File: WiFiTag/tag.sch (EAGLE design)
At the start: 65 parts, among them IC2 MCP73831/OT, U2 CP2104-F03-GM

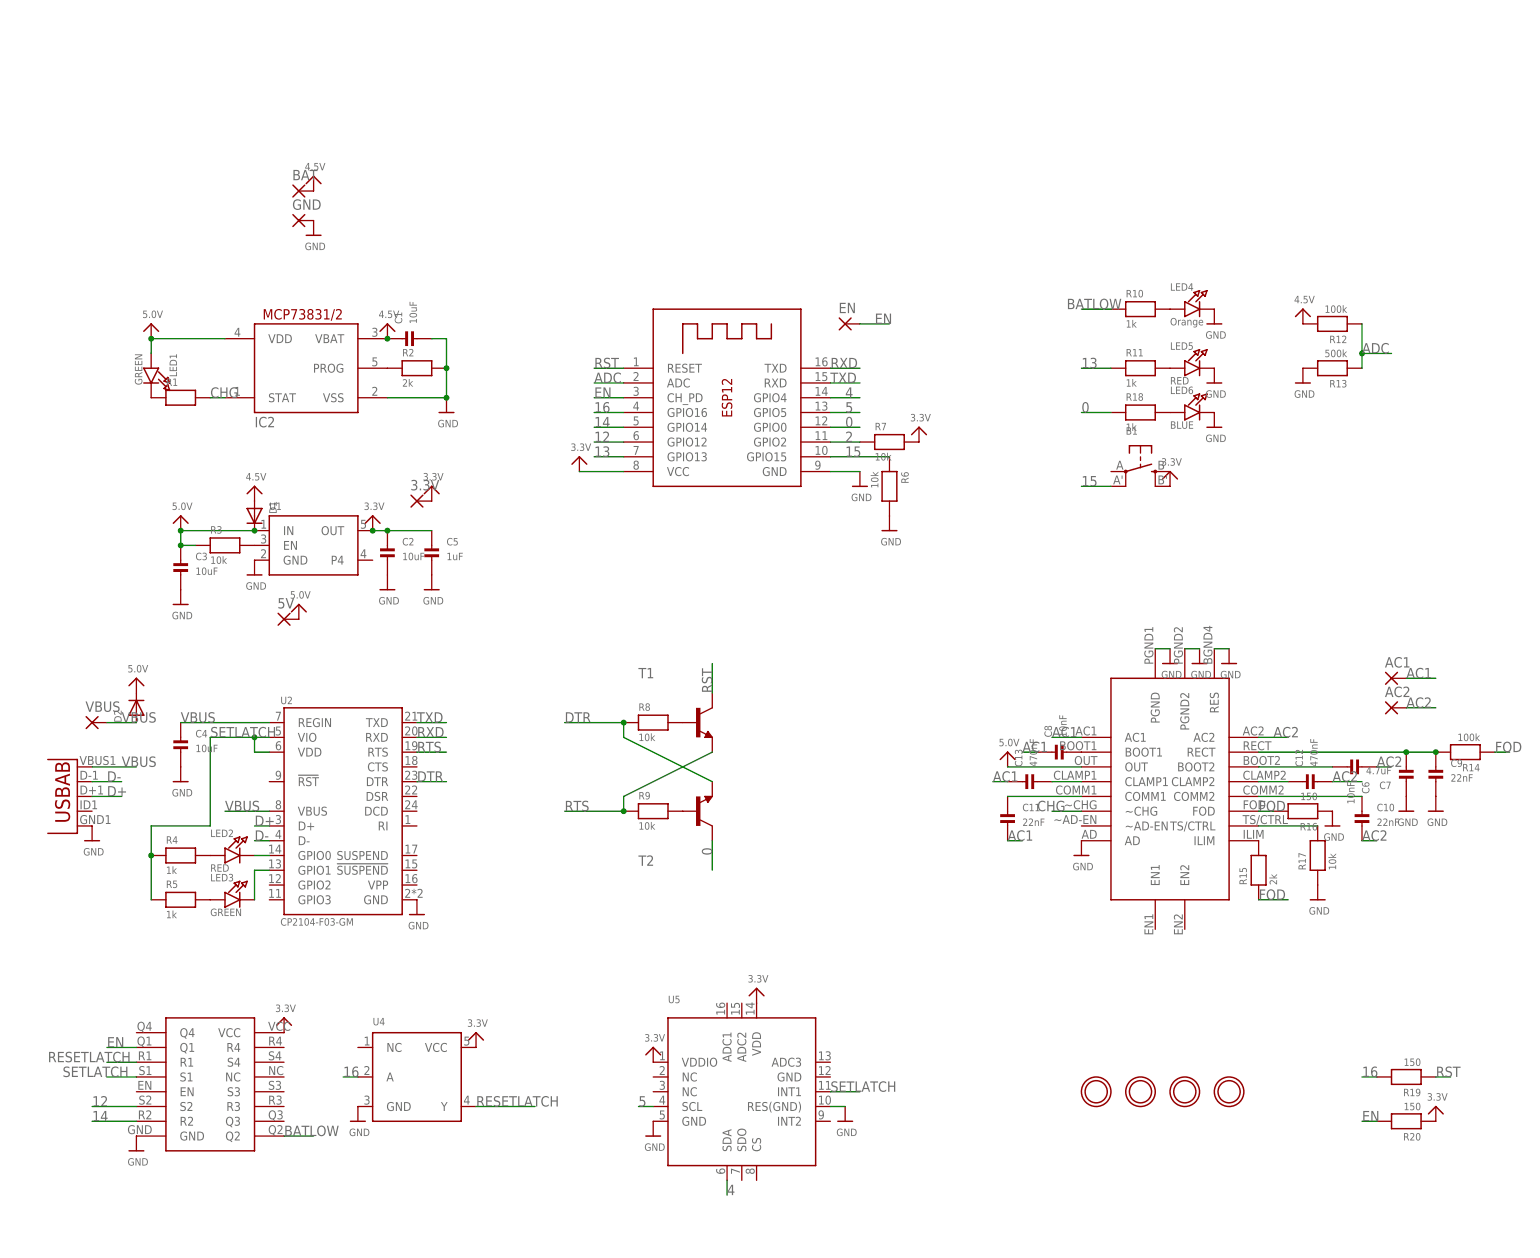
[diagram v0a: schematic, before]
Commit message: WifiTagV0.4
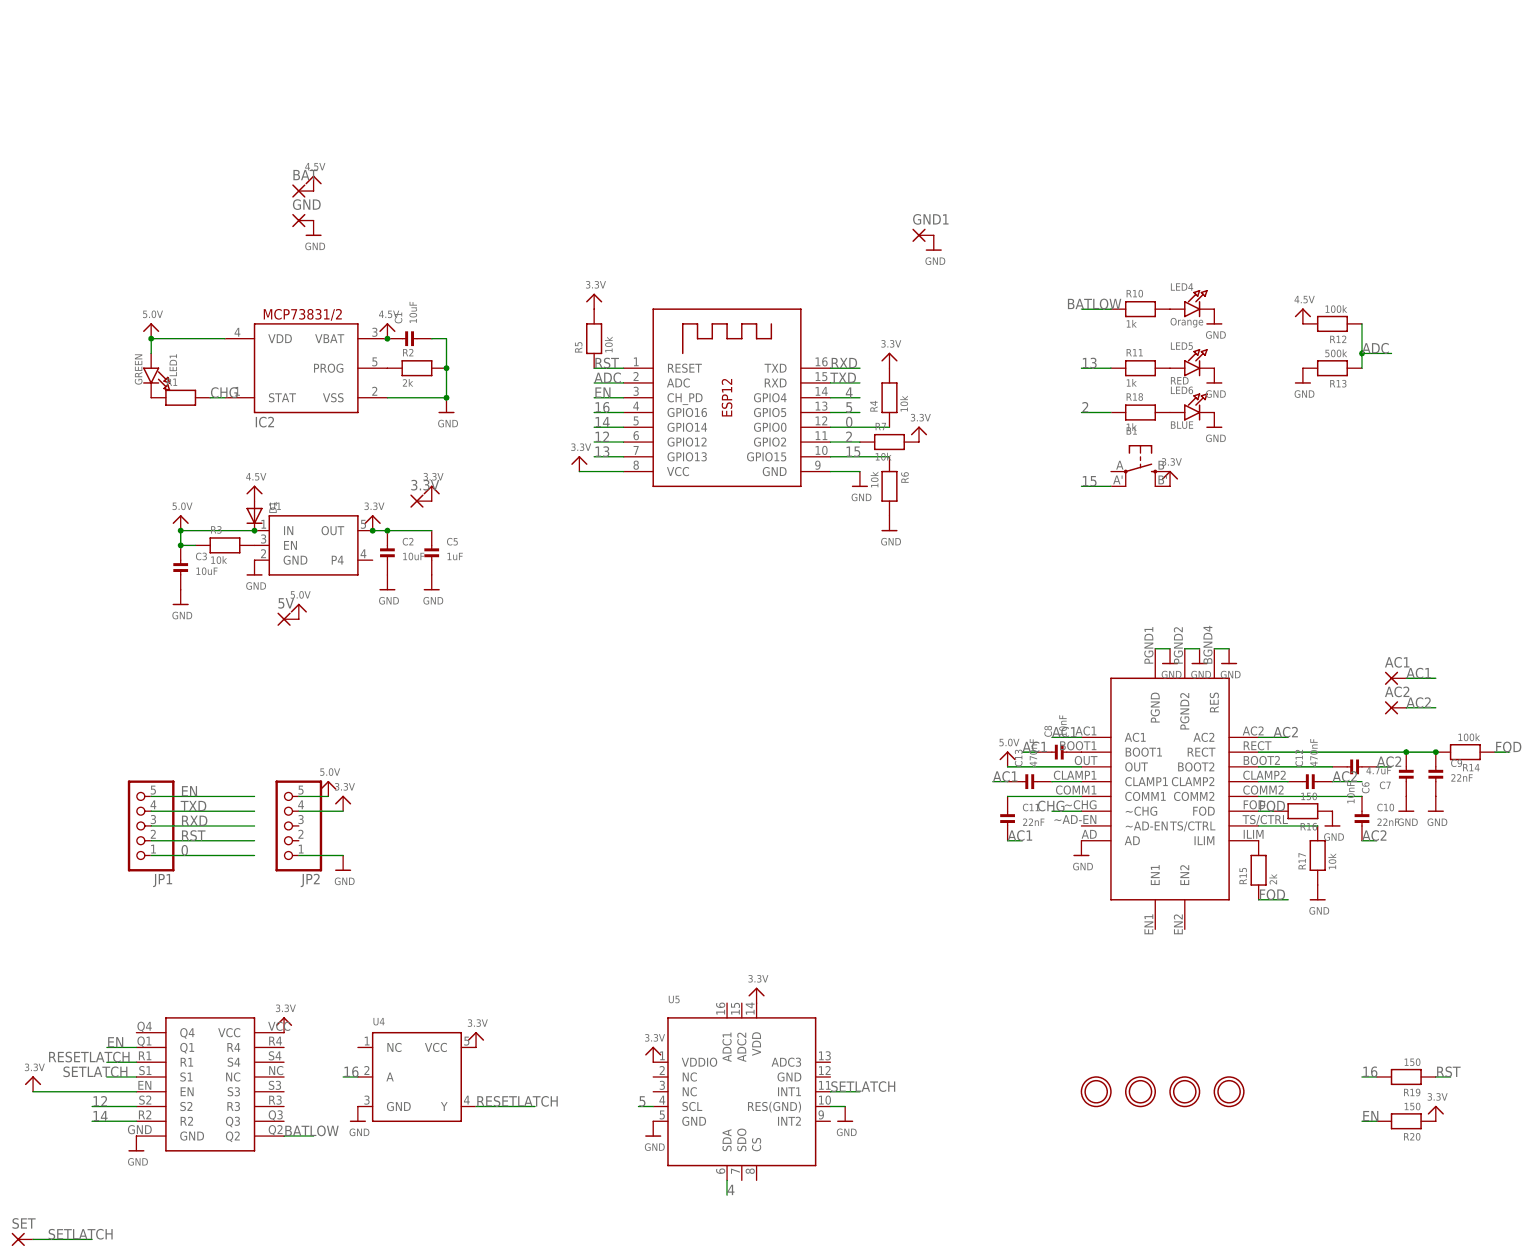
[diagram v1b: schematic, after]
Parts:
- removed C4: 10uF, microbuilder:CAP_CERAMIC0603
- removed D2: (no value), adafruit:DIODESOD-123
- removed EN, VBUS: (no value), wirepad:SMD2
- removed LED2: RED, microbuilder:LED0603
- removed LED3: GREEN, microbuilder:LED0603
- removed R8, R9: 10k, microbuilder:RESISTOR0402
- removed T1, T2: (no value), transistor:MMBT2222ALT1-NPN-SOT23-BEC
- removed U2: CP2104-F03-GM, Silicon Labs:CP2104-F03-GM
- removed U3: (no value), MicroUSB:USB""
- added GND1, SET: (no value), wirepad:SMD2
- added JP1, JP2: (no value), pinhead:PINHD-1X55X2MM
- R4, R5: value 1k -> 10k
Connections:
- removed net D+: U2.D+, U3.D+
- removed net D-: U2.D-, U3.D-
- removed net DTR: R8.1, T2.E, U2.DTR
- removed net N$10: R8.2, T1.B
- removed net N$11: R9.2, T2.B
- removed net N$6: LED2.A, R4.2
- removed net N$7: LED3.A, R5.2
- removed net N$8: LED2.C, U2.GPIO0
- removed net N$9: LED3.C, U2.GPIO1
- removed net RTS: R9.1, T1.E, U2.RTS
- removed net VBUS: C4.P$1, D2.A, U2.REGIN, U2.VBUS, U3.VBUS, VBUS.P
- net 0: now also JP1.1, R4.1; no longer R18.1, T2.C
- net 2: now also R18.1
- net 3.3V: now also JP2.4, R4.2, R5.2, U$24.EN
- net 5.0V: now also JP2.5; no longer D2.C
- net EN: now also JP1.5; no longer EN.P
- net GND: now also GND1.P, JP2.1; no longer C4.P$2, U2.GND, U3.GND
- net RST: now also JP1.2, R5.1; no longer T1.C
- net RXD: now also JP1.3; no longer U2.RXD
- net SETLATCH: now also SET.P; no longer R4.1, R5.1, U2.VDD, U2.VIO
- net TXD: now also JP1.4; no longer U2.TXD
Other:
- moved on the sheet: R4, R5

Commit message: new tag version 0.5
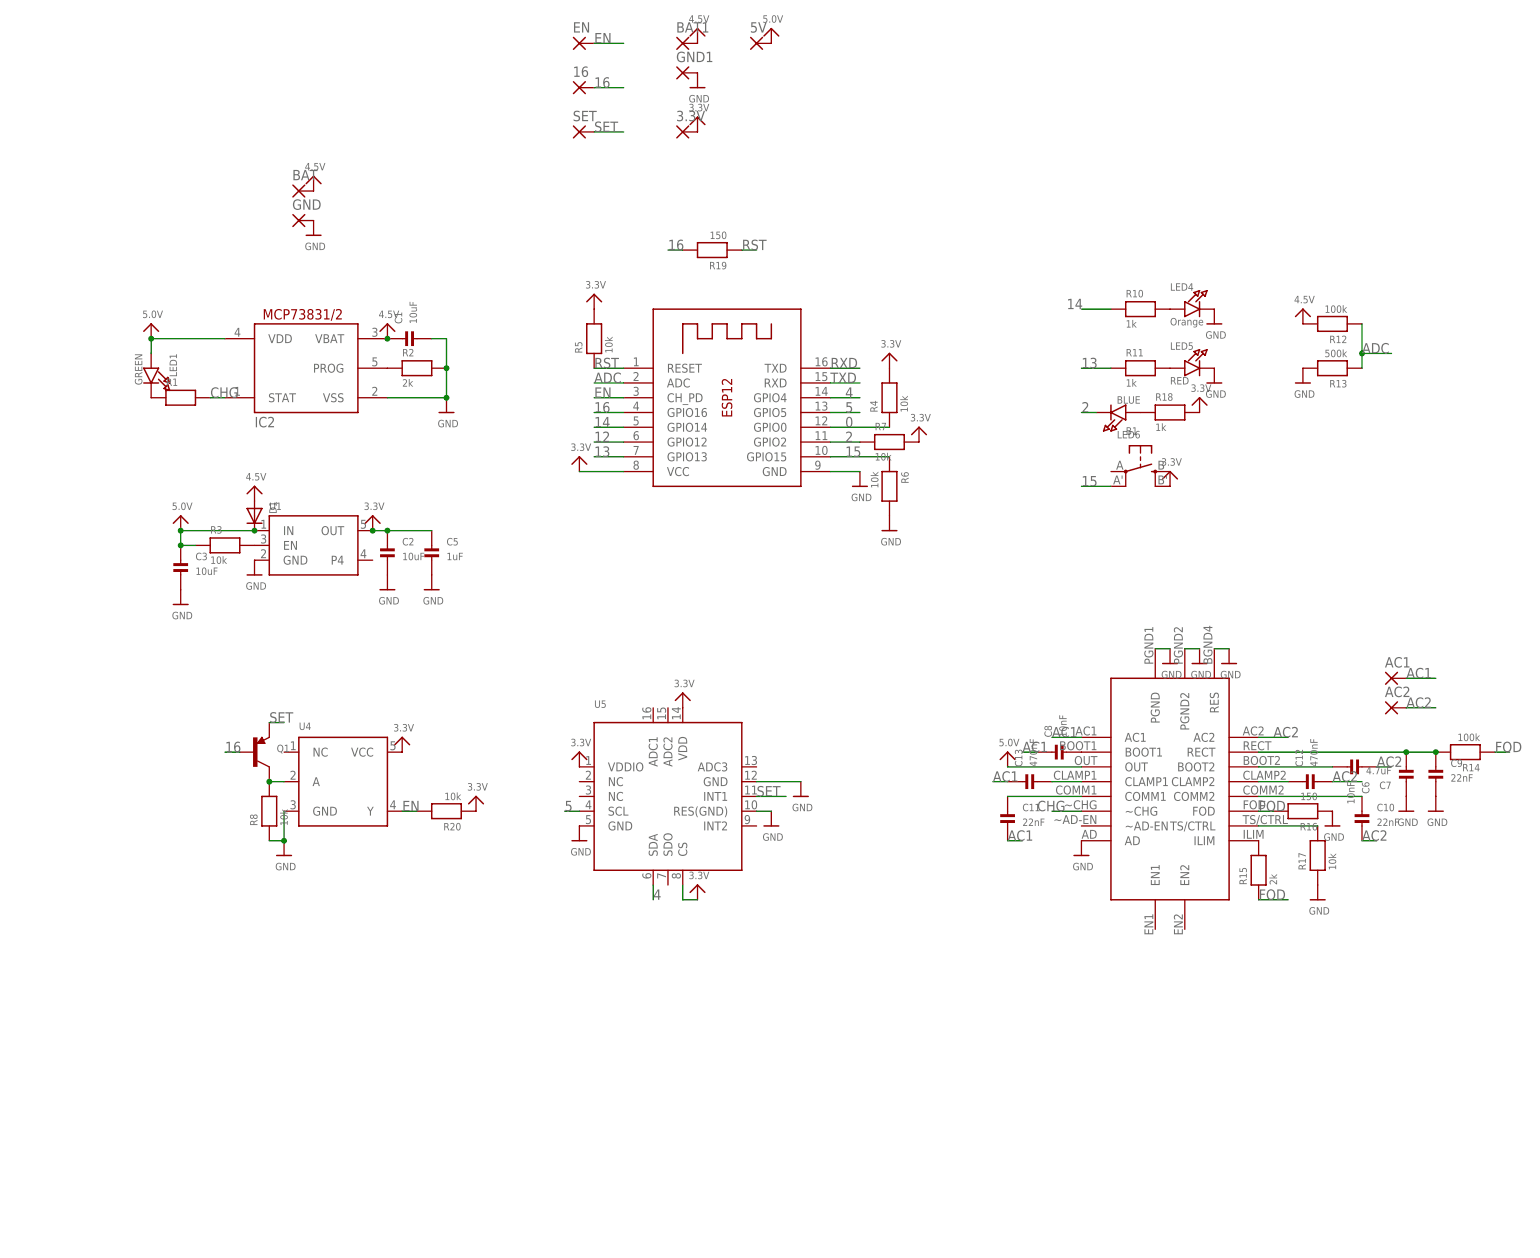
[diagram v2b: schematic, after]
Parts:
- removed JP1, JP2: (no value), pinhead:PINHD-1X55X2MM
- removed U$21, U$47, U$48, U$49: MOUNTINGHOLE2.5, microbuilder:MOUNTINGHOLE2.5
- removed U$24: CD4043B, masterthesis:CD4043B
- added 16, BAT1, EN: (no value), wirepad:SMD2
- added Q1: (no value), microbuilder:TRANSISTOR_PNPSOT23-REFLOW
- added R8: 10k, microbuilder:RESISTOR0402
- R20: value 150 -> 10k
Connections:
- removed net BATLOW: R10.1, U$24.Q2
- removed net RESETLATCH: U$24.R1, U4.Y
- removed net SETLATCH: SET.P, U$24.S1, U5.INT1
- new net N$6: Q1.C, R8.2, U4.A
- new net SET: Q1.E, SET.P, U5.INT1
- net 0: no longer JP1.1
- net 12: no longer U$24.S2
- net 14: now also R10.1; no longer U$24.R2
- net 16: now also 16.P, Q1.B; no longer U4.A
- net 2: now also LED6.C; no longer R18.1
- net 3.3V: now also R18.2, U5.CS; no longer JP2.4, U$24.EN, U$24.VCC
- net 4.5V: now also BAT1.P
- net 5.0V: no longer JP2.5
- net EN: now also EN.P, U4.Y; no longer JP1.5, U$24.Q1
- net GND: now also R8.1, U5.GND@2; no longer JP2.1, LED6.C, U$24.GND
- net N$4: now also R18.1; no longer R18.2
- net RST: no longer JP1.2
- net RXD: no longer JP1.3
- net TXD: no longer JP1.4
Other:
- moved on the sheet: 3.3V, 5V, GND1, LED6, R18, R19, R20, SET, U4, U5
